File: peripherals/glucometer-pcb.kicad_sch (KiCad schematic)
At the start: 10 parts, among them U1 ESP32_DevKit_V1_DOIT

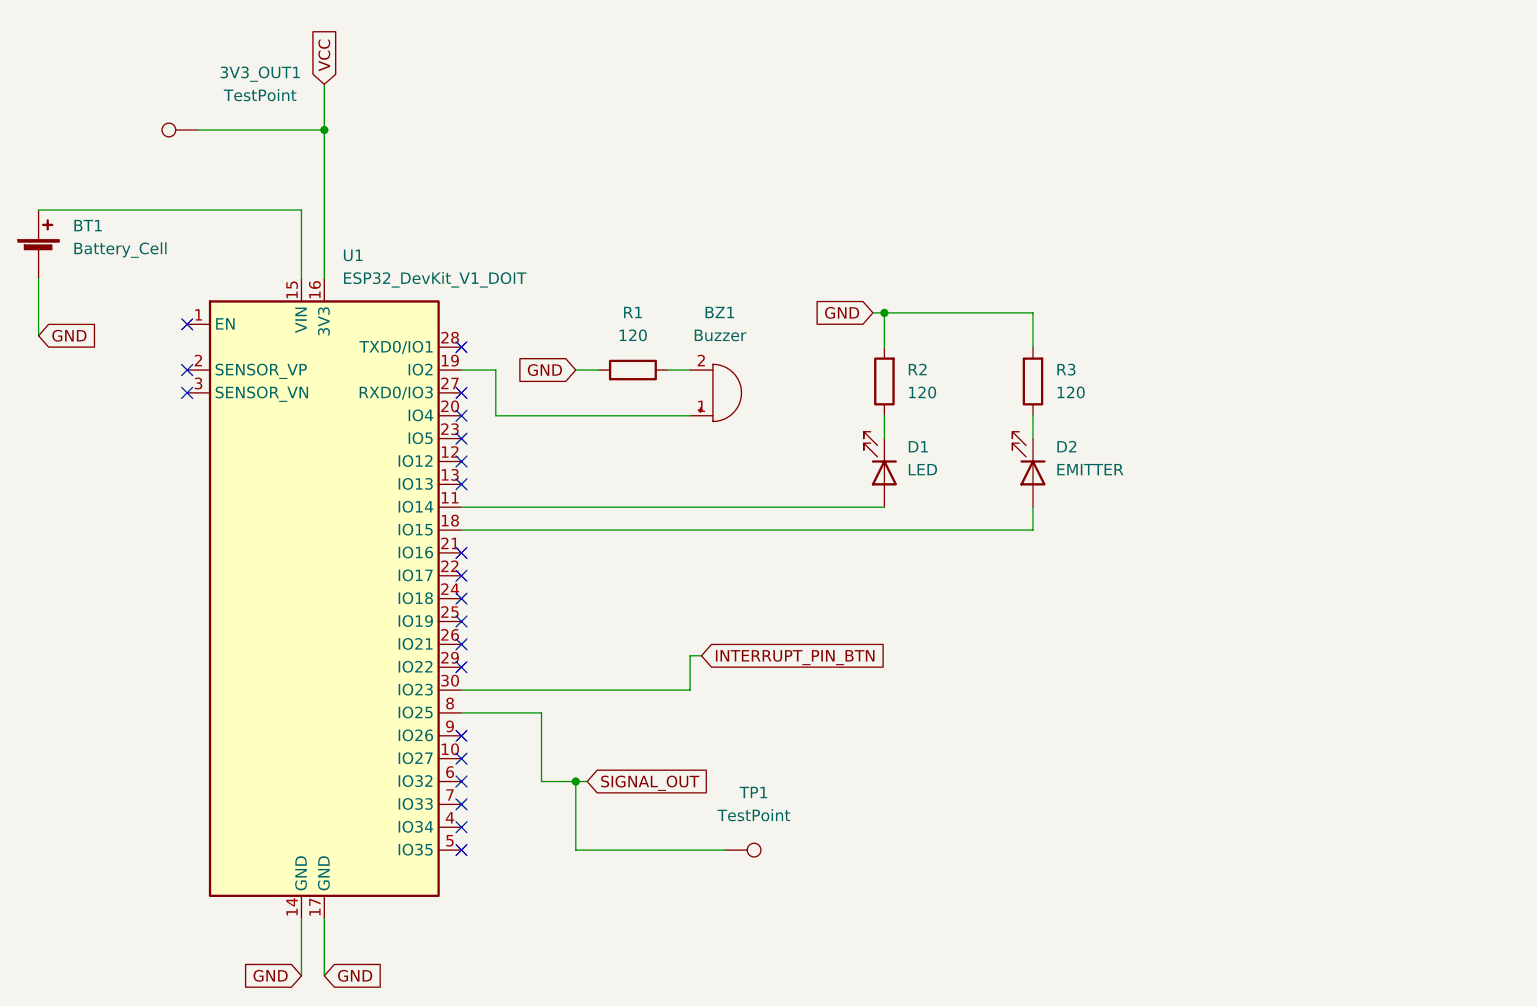
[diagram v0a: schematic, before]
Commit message: fixed PCB
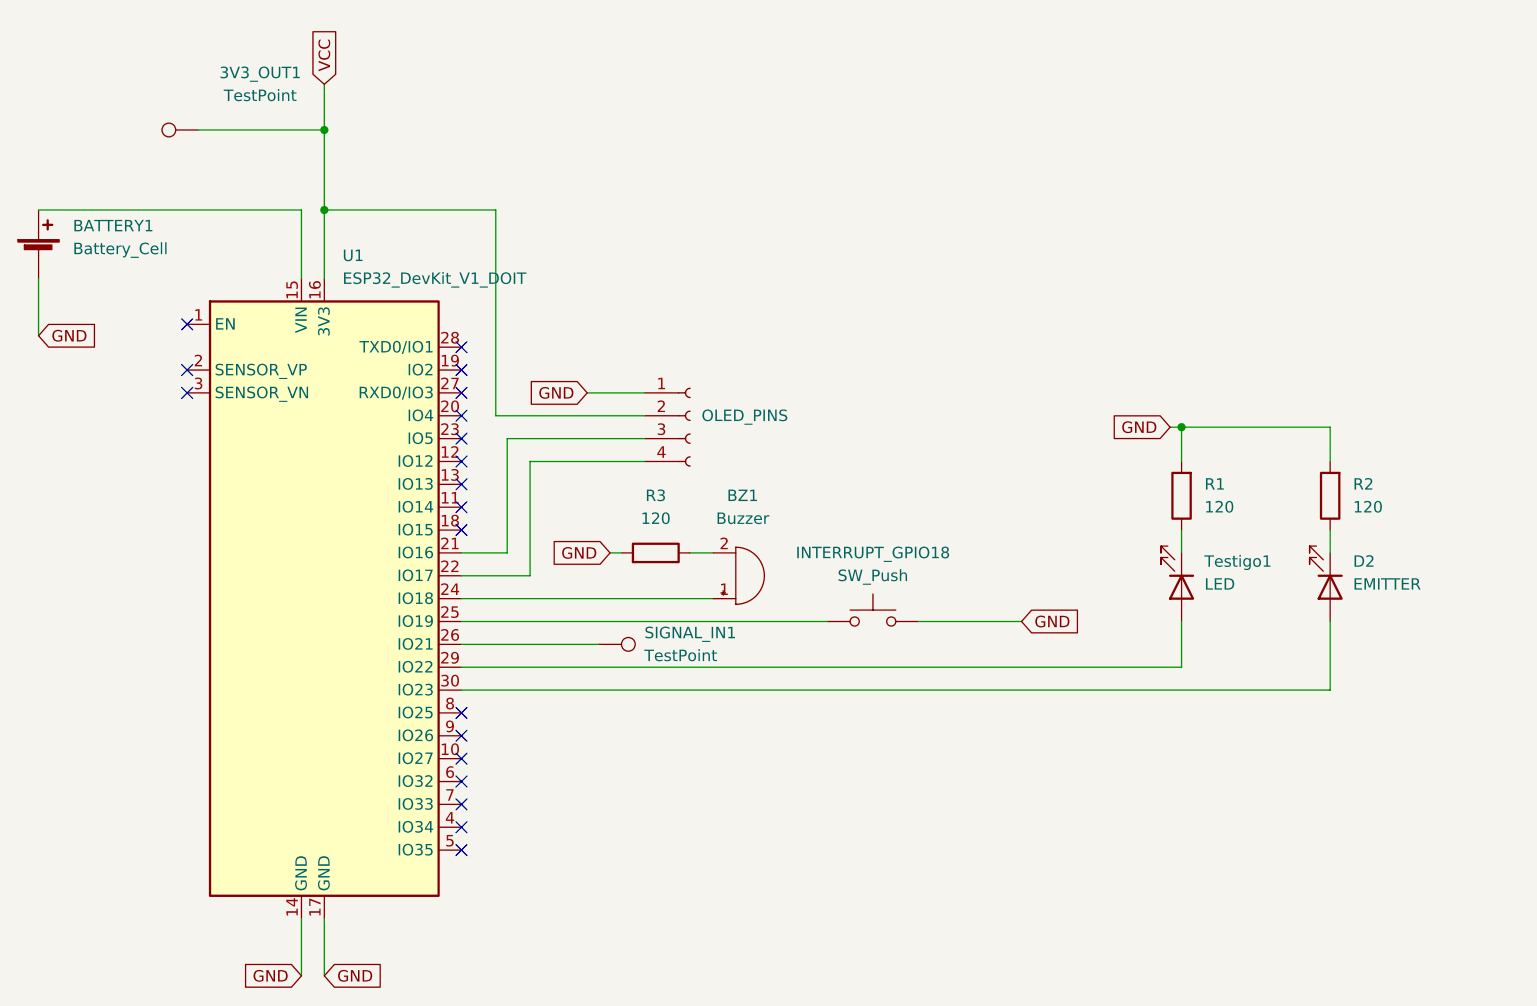
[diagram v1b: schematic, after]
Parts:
- added INTERRUPT_GPIO18: SW_Push, symbol Switch:SW_Push
- added OLED_PINS: (no value), symbol Connector:Conn_01x04_Female
- renumbered BT1 to BATTERY1, R2 to R1, R3 to R2, R1 to R3, TP1 to SIGNAL_IN1, D1 to Testigo1
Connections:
- net INTERRUPT_PIN_BTN is gone; now on an unnamed net: U1.30 (IO23)
- net GND: now also INTERRUPT_GPIO18.2, OLED_PINS.1 (Pin_1)
- net VCC: now also OLED_PINS.2 (Pin_2)
- net at Testigo1.2 (A): now also U1.29 (IO22); no longer U1.11 (IO14)
- net at D2.2 (A): no longer U1.18 (IO15)
- net at BZ1.1 (-): now also U1.24 (IO18); no longer U1.19 (IO2)
- net at U1.21 (IO16): now also OLED_PINS.3 (Pin_3)
- net at U1.22 (IO17): now also OLED_PINS.4 (Pin_4)
- net at U1.25 (IO19): now also INTERRUPT_GPIO18.1
- net at U1.26 (IO21): now also SIGNAL_IN1.1
- net SIGNAL_OUT: no longer names the net of U1.8 (IO25)
- net SIGNAL_OUT: no longer SIGNAL_IN1.1
- no-connect marks 21 -> 19
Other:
- moved on the sheet: BZ1, D2, R1, R2, R3, SIGNAL_IN1, Testigo1

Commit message: changes
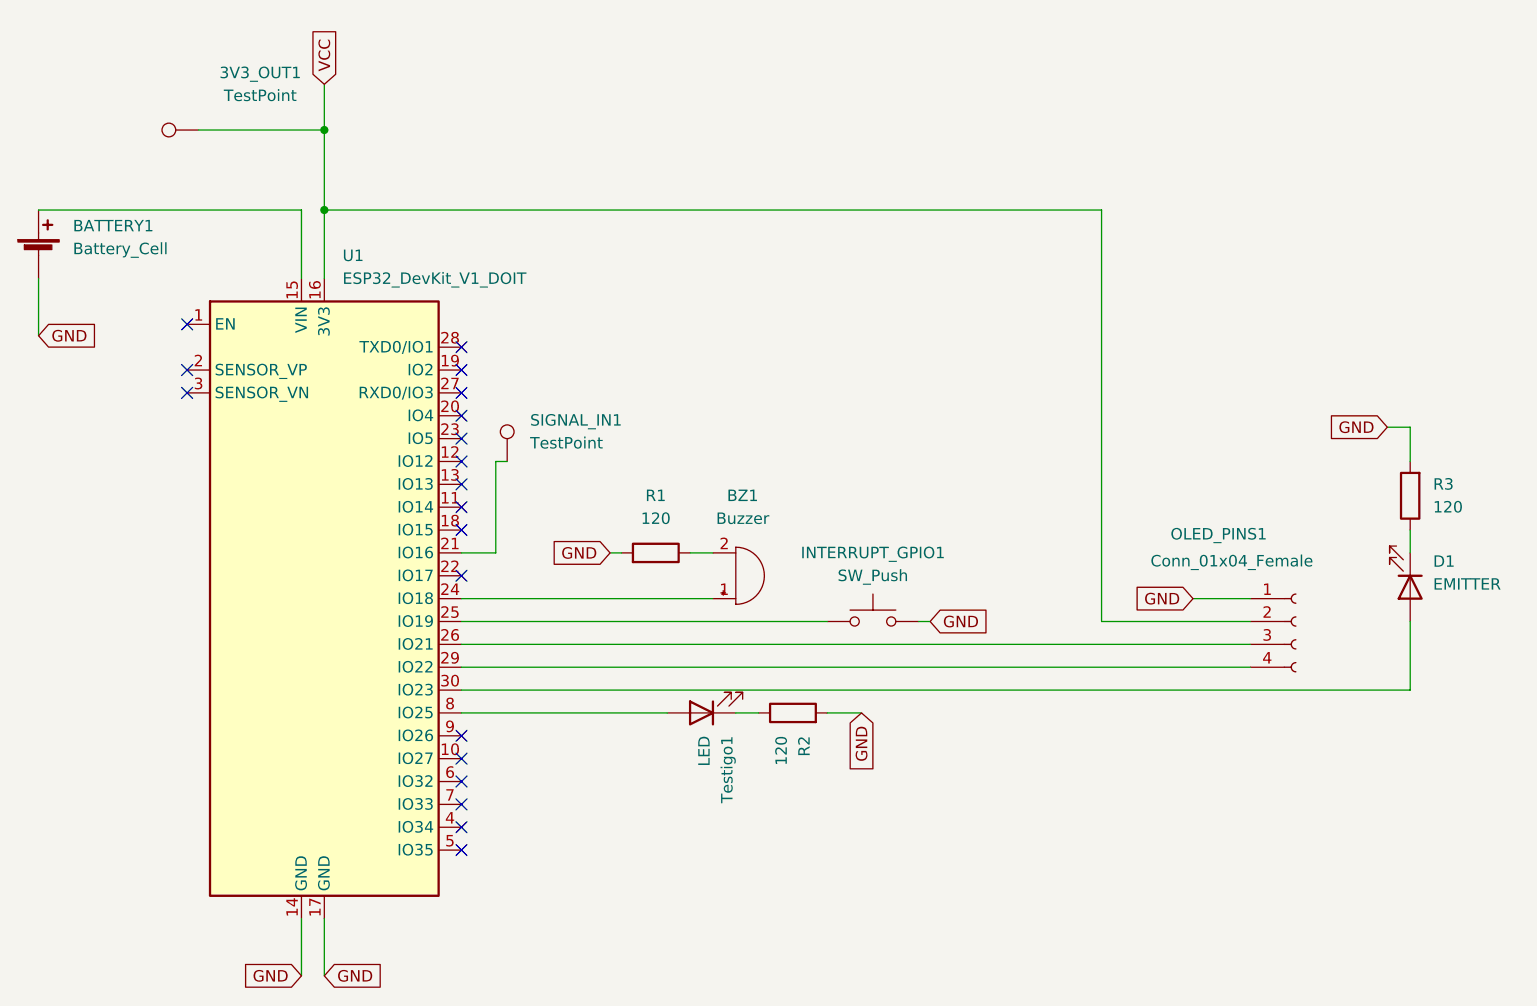
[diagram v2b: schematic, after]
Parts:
- INTERRUPT_GPIO1: renamed from INTERRUPT_GPIO18; footprint (none) -> Connector_Wire:SolderWire-0.1sqmm_1x02_P3.6mm_D0.4mm_OD1mm
- OLED_PINS1: renamed from OLED_PINS; value (none) -> Conn_01x04_Female; footprint (none) -> Connector_Wire:SolderWire-0.1sqmm_1x04_P3.6mm_D0.4mm_OD1mm
- renumbered D2 to D1, R3 to R1, R1 to R2, R2 to R3
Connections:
- net at Testigo1.2 (A): now also U1.8 (IO25); no longer U1.29 (IO22)
- net at OLED_PINS1.3 (Pin_3): now also U1.26 (IO21); no longer U1.21 (IO16)
- net at OLED_PINS1.4 (Pin_4): now also U1.29 (IO22); no longer U1.22 (IO17)
- net at SIGNAL_IN1.1: now also U1.21 (IO16); no longer U1.26 (IO21)
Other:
- moved on the sheet: D1, OLED_PINS1, R2, R3, SIGNAL_IN1, Testigo1
